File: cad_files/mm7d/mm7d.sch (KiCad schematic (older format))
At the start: 24 parts, among them P1 BNC, P2 DB9, U1 Adafruit Huzzah Breakout, U2 MQ-135M, U3 DHT11

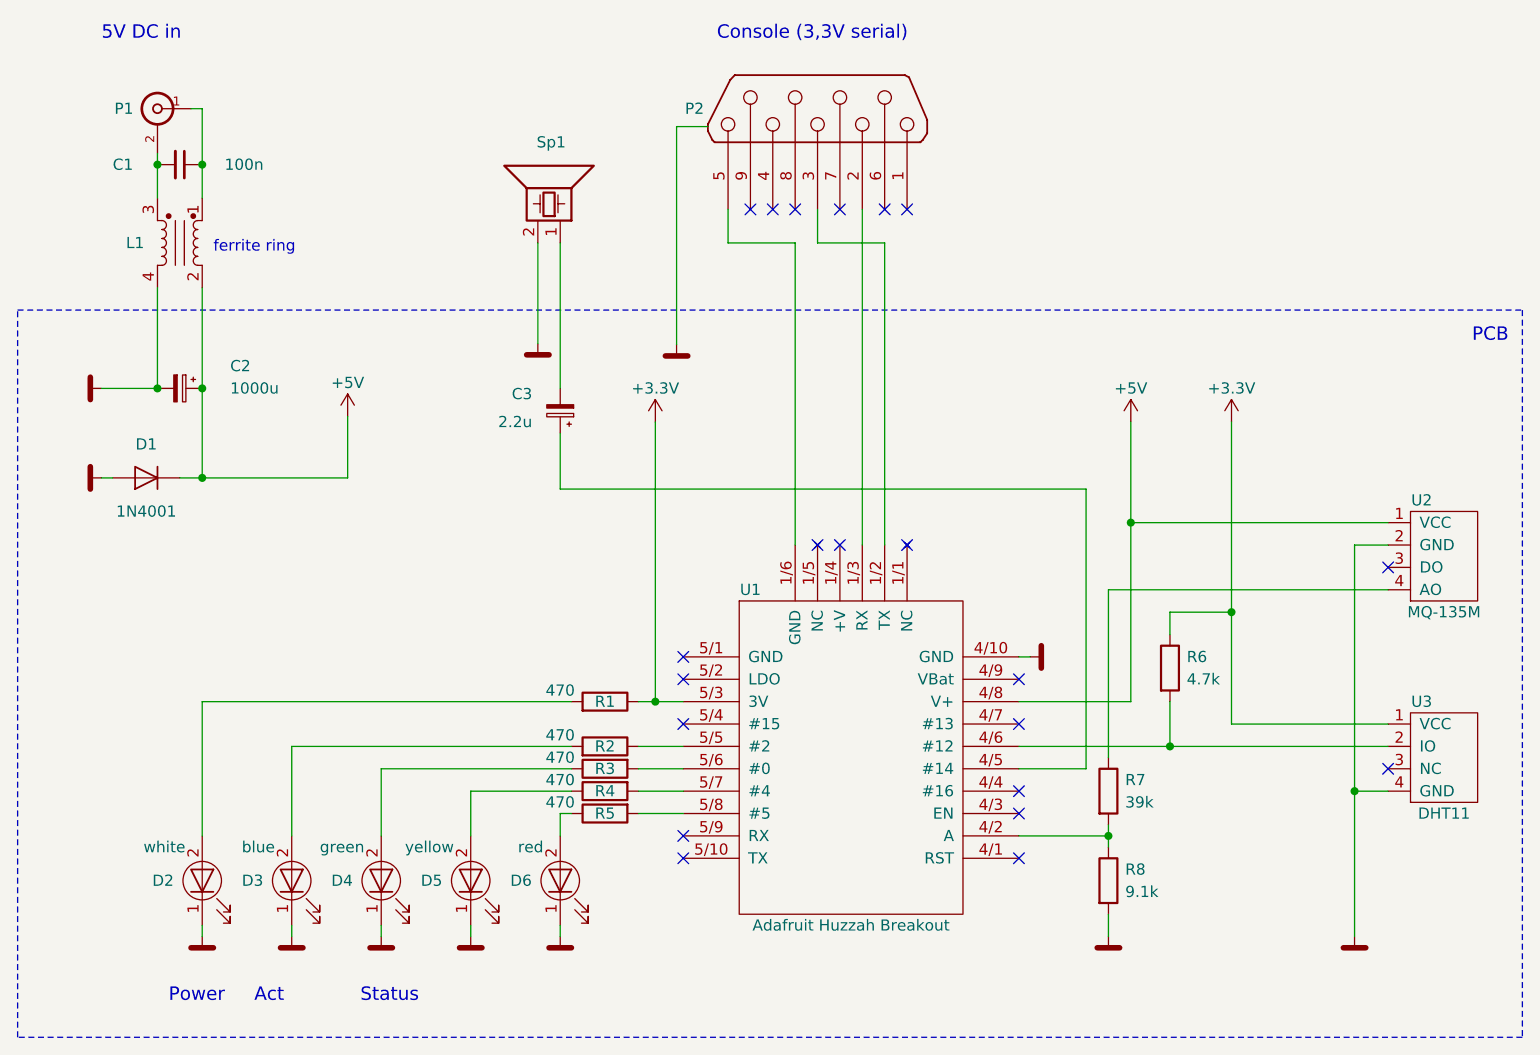
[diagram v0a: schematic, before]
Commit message: 200714
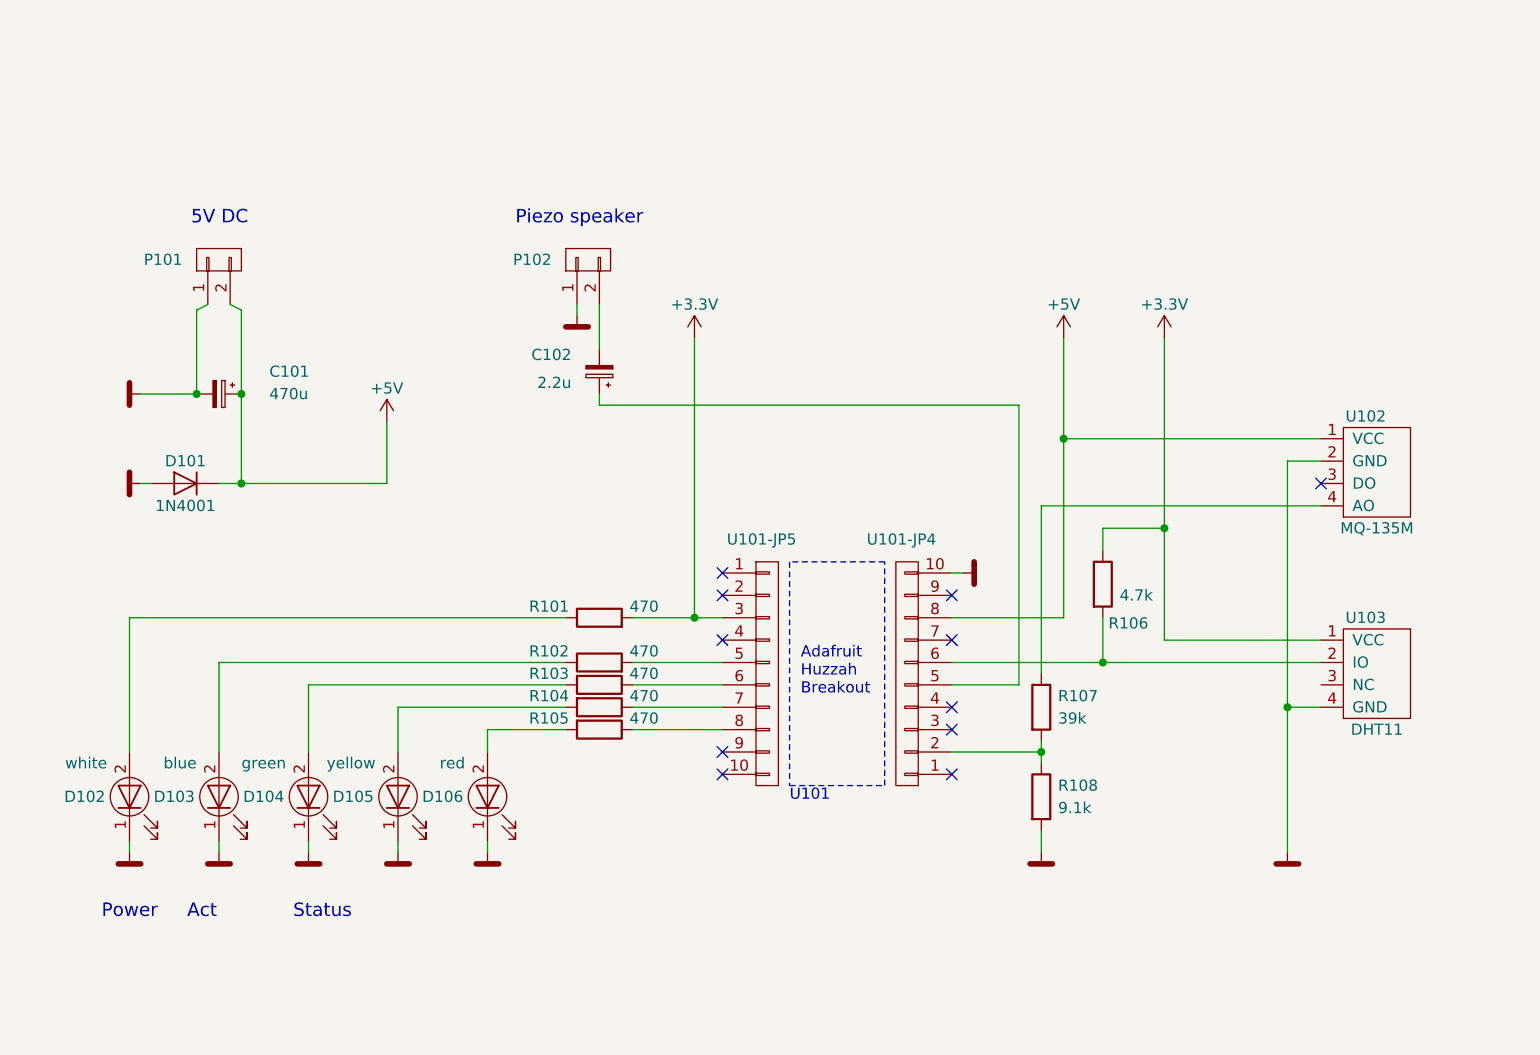
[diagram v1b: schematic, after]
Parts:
- removed C1: 100n, symbol device:C_Small
- removed D1: 1N4001, symbol pzs_others:diode
- removed L1: EMI_Filter_LL, symbol device:EMI_Filter_LL
- removed P1: BNC, symbol mm7d-rescue:BNC
- removed P2: DB9, symbol mm7d-rescue:DB9
- removed Sp1: Speaker Crystal, symbol device:Speaker_Ultrasound
- removed U1: Adafruit Huzzah Breakout, symbol pzs_devices:Adafruit_Huzzah_Breakout
- added D101: 1N4001, Diodes_THT:Diode_DO-41_SOD81_Horizontal_RM10, symbol D
- added P101, P102: CONN_01X02, Socket_Strips:Socket_Strip_Straight_1x02, symbol CONN_01X02
- added U101-JP4, U101-JP5: CONN_01X10, Socket_Strips:Socket_Strip_Straight_1x10, symbol CONN_01X10
- C101: renamed from C2; value 1000u -> 470u; footprint (none) -> Capacitors_THT:C_Radial_D8_L11.5_P3.5
- C102: renamed from C3; footprint (none) -> Capacitors_THT:C_Rect_L7_W4.5_P5
- D102: renamed from D2; footprint (none) -> LEDs:LED-3MM
- D103: renamed from D3; footprint (none) -> LEDs:LED-3MM
- D104: renamed from D4; footprint (none) -> LEDs:LED-3MM
- D105: renamed from D5; footprint (none) -> LEDs:LED-3MM
- D106: renamed from D6; footprint (none) -> LEDs:LED-3MM
- R101: renamed from R1; footprint (none) -> Resistors_THT:Resistor_Horizontal_RM7mm
- R102: renamed from R2; footprint (none) -> Resistors_THT:Resistor_Horizontal_RM7mm
- R103: renamed from R3; footprint (none) -> Resistors_THT:Resistor_Horizontal_RM7mm
- R104: renamed from R4; footprint (none) -> Resistors_THT:Resistor_Horizontal_RM7mm
- R105: renamed from R5; footprint (none) -> Resistors_THT:Resistor_Horizontal_RM7mm
- R106: renamed from R6; footprint (none) -> Resistors_THT:Resistor_Horizontal_RM7mm
- R107: renamed from R7; footprint (none) -> Resistors_THT:Resistor_Horizontal_RM10mm
- R108: renamed from R8; footprint (none) -> Resistors_THT:Resistor_Horizontal_RM10mm
- U102: renamed from U2; footprint (none) -> Socket_Strips:Socket_Strip_Straight_1x04
- U103: renamed from U3; footprint (none) -> Socket_Strips:Socket_Strip_Straight_1x04
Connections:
- net +3V3: now also R101.2, U101-JP5.3 (P3); no longer R101.1
- net +5V: now also D101.1 (K), P101.2 (P2), U101-JP4.8 (P8)
- net GND: now also D101.2 (A), P101.1 (P1), P102.1 (P1), U101-JP4.10 (P10)
- net at R107.2, R108.1: now also U101-JP4.2 (P2)
- net at C102.1: now also U101-JP4.5 (P5)
- net at R106.2, U103.2 (IO): now also U101-JP4.6 (P6)
- net at R102.1: now also D103.2 (A)
- net at R103.2: now also D104.2 (A)
- net at R104.2: now also D105.2 (A)
- net at R105.2: now also D106.2 (A)
- net at R103.1: now also U101-JP5.6 (P6); no longer D104.2 (A)
- net at R104.1: now also U101-JP5.7 (P7); no longer D105.2 (A)
- net at R105.1: now also U101-JP5.8 (P8); no longer D106.2 (A)
- net at R102.2: now also U101-JP5.5 (P5); no longer D103.2 (A)
- net at D102.2 (A): now also R101.1; no longer R101.2
- net at C102.2: now also P102.2 (P2)
- no-connect marks 21 -> 11
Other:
- note added: "5V DC"
- note added: "Adafruit\nHuzzah\nBreakout"
- note added: "Piezo speaker"
- note added: "U101"
- note removed: "5V DC in"
- note removed: "Console (3,3V serial)"
- note removed: "PCB"
- note removed: "ferrite ring"
- moved on the sheet: C101, C102, D102, D103, D104, D105, D106, R101, R102, R103, R104, R105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
